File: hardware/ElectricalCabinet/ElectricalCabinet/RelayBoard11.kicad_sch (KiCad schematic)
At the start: 0 parts

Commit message: Further wiring updates
Populated 6100 Bus
Corrected number of relay boards
Added 110v outputs to relay boards and noted light positon
Uploaded light scheme to documents folder
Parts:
- added C11: 0.1uF, Capacitor_SMD:C_0805_2012Metric, symbol Device:C
- added D81, D82, D83, D84, D85, D86, D87, D88: LED, LED_SMD:LED_0805_2012Metric, symbol Device:LED
- added J22: Screw_Terminal_01x06, TerminalBlock:TerminalBlock_MaiXu_MX126-5.0-06P_1x06_P5.00mm, symbol Connector:Screw_Terminal_01x06
- added J23: Screw_Terminal_01x09, TerminalBlock:TerminalBlock_MaiXu_MX126-5.0-09P_1x09_P5.00mm, symbol Connector:Screw_Terminal_01x09
- added K81, K82, K83, K84, K85, K86, K87, K88: G3MB-202P DC5, TrafficLightLibrary:G3MB_202P_DC5, symbol TrafficLightLibrary:G3MB-202P_DC5
- added R81, R82, R83, R84, R85, R86, R87, R88: 1kΩ, Resistor_SMD:R_0805_2012Metric, symbol Device:R
- added U12: TPIC6B595N, TrafficLightLibrary:TPIC6B595N, symbol TrafficLightLibrary:TPIC6B595N
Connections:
- new net: J23.9 (Pin_9), K81.1, K82.1, K83.1, K84.1, K85.1, K86.1, K87.1, K88.1
- new net: J23.7 (Pin_7), K87.2
- new net: D81.2 (A), D82.2 (A), D83.2 (A), D84.2 (A), D85.2 (A), D86.2 (A), D87.2 (A), D88.2 (A), K81.3, K82.3, K83.3, K84.3, K85.3, K86.3, K87.3, K88.3
- new net: K87.4, R87.2, U12.16 (DRAIN6)
- new net: J23.5 (Pin_5), K85.2
- new net: K85.4, R85.2, U12.14 (DRAIN4)
- new net: D85.1 (K), R85.1
- new net: J23.1 (Pin_1), K81.2
- new net: J23.2 (Pin_2), K82.2
- new net: J23.3 (Pin_3), K83.2
- new net: J23.4 (Pin_4), K84.2
- new net: J23.6 (Pin_6), K86.2
- new net: J23.8 (Pin_8), K88.2
- new net: D86.1 (K), R86.1
- new net: K86.4, R86.2, U12.15 (DRAIN5)
- new net: K88.4, R88.2, U12.17 (DRAIN7)
- new net: C11.1, J22.2 (Pin_2), U12.10 (GND), U12.11 (GND), U12.19 (GND), U12.9 (~{G})
- new net: C11.2, J22.6 (Pin_6), U12.2 (VCC), U12.8 (~{SRCLR})
- new net: K82.4, R82.2, U12.5 (DRAIN1)
- new net: K84.4, R84.2, U12.7 (DRAIN3)
- new net: D84.1 (K), R84.1
- new net: J22.1 (Pin_1), U12.18 (SEROUT)
- new net: J22.3 (Pin_3), U12.13 (SRCK)
- new net: J22.4 (Pin_4), U12.12 (RCK)
- new net: D83.1 (K), R83.1
- new net: D88.1 (K), R88.1
- new net: K81.4, R81.2, U12.4 (DRAIN0)
- new net: K83.4, R83.2, U12.6 (DRAIN2)
- new net: D81.1 (K), R81.1
- new net: D87.1 (K), R87.1
- new net: D82.1 (K), R82.1
- new net SERIN: J22.5 (Pin_5), U12.3 (SERIN)
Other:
- note added: "RELAY MODULE 11"

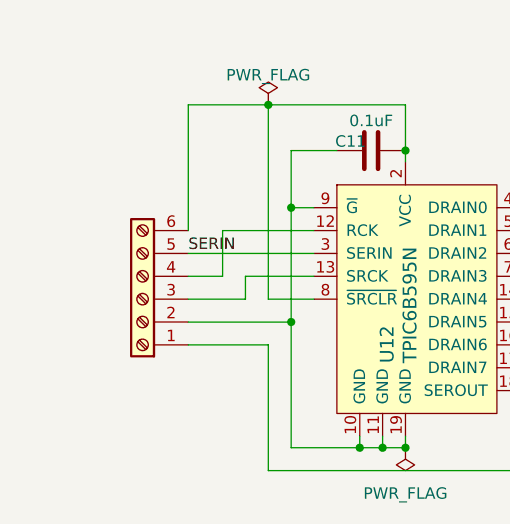
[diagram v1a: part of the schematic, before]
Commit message: Electrical Cabinet done
Electrical Cabinet done, let me know if there are any changes or mistakes.
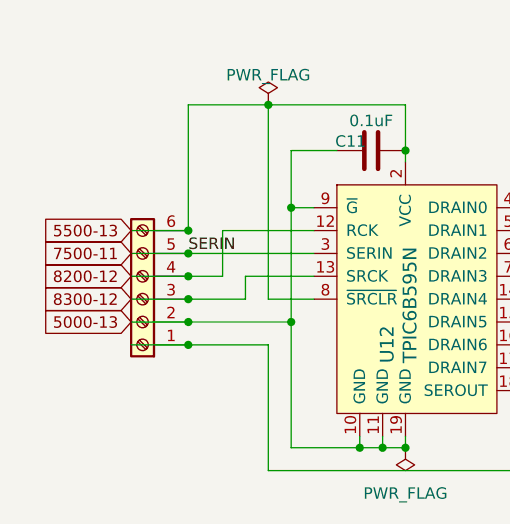
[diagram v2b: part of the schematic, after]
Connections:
- net 5000-13: now reaches C11.1, J22.2 (Pin_2), U12.10 (GND), U12.11 (GND), U12.19 (GND), U12.9 (~{G})
- net 5500-13: now reaches C11.2, J22.6 (Pin_6), U12.2 (VCC), U12.8 (~{SRCLR})
- net 8300-12: now reaches J22.3 (Pin_3), U12.13 (SRCK)
- net 8200-12: now reaches J22.4 (Pin_4), U12.12 (RCK)
- net SERIN renamed 7500-11
